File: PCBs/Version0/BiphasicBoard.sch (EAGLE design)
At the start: 11 parts

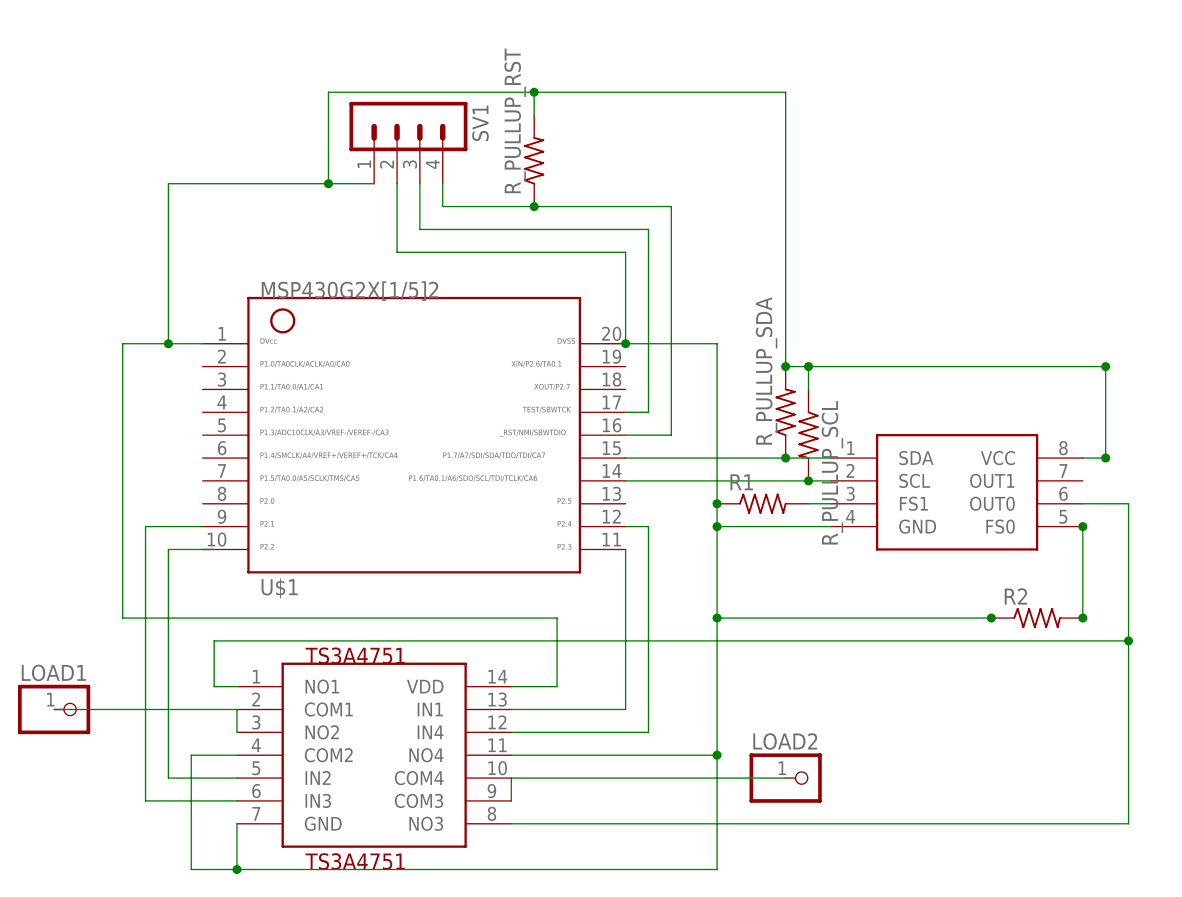
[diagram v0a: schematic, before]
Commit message: Updated Library Parts
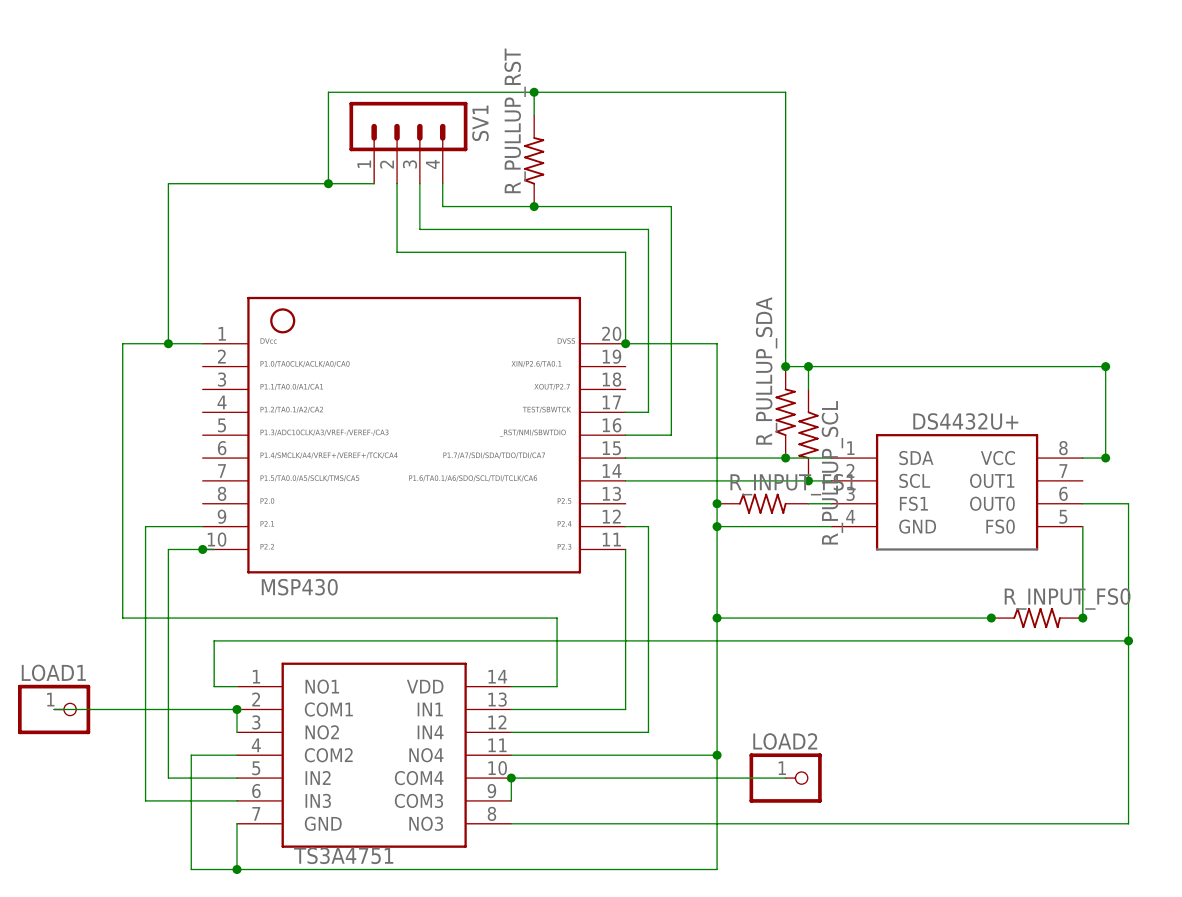
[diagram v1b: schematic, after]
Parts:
- removed DS4432: (no value), DS4432U+:DS4432U+
- removed R1, R2: (no value), resistor:R-US_R0603
- removed U$1: G2X[1/5]2---PW20, TI_MSP430_v16:G2X[1/5]2---PW20
- added DS4432U+: (no value), BiphasicBoard:DS4432U+
- added MSP430: (no value), BiphasicBoard:MSP430
- added R_INPUT_FS0, R_INPUT_FS1: (no value), BiphasicBoard:R-US_R0603
- LOAD1, LOAD2: device pinhead:PINHD-1X1 -> BiphasicBoard:PINHD-1X1
- R_PULLUP_RST, R_PULLUP_SCL, R_PULLUP_SDA: device resistor:R-US_R0603 -> BiphasicBoard:R-US_R0603
- SV1: device con-lstb:MA04-1 -> BiphasicBoard:MA04-1
- TS3A4751: device TS3A4751:TS3A4751 -> BiphasicBoard:TS3A4751
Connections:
- removed net N$10: TS3A4751.IN1, U$1.11
- removed net N$11: TS3A4751.IN4, U$1.12
- new net IN1: MSP430.11, TS3A4751.IN1
- new net IN4: MSP430.12, TS3A4751.IN4
- net CURRENT0: now also DS4432U+.OUT0; no longer DS4432.OUT0
- net GND: now also DS4432U+.GND, MSP430.20, R_INPUT_FS0.1, R_INPUT_FS1.1; no longer DS4432.GND, R1.1, R2.1, U$1.20
- net N$1: now also DS4432U+.SCL, MSP430.14; no longer DS4432.SCL, U$1.14
- net N$2: now also DS4432U+.SDA, MSP430.15; no longer DS4432.SDA, U$1.15
- net N$4: now also MSP430.10; no longer U$1.10
- net N$8: now also DS4432U+.FS0, R_INPUT_FS0.2; no longer DS4432.FS0, R2.2
- net N$9: now also MSP430.9; no longer U$1.9
- net TEST: now also MSP430.17; no longer U$1.17
- net VDD: now also DS4432U+.VCC, MSP430.1; no longer DS4432.VCC, U$1.1
- net VIA1: now also DS4432U+.FS1, R_INPUT_FS1.2; no longer DS4432.FS1, R1.2
- net _RST: now also MSP430.16; no longer U$1.16
